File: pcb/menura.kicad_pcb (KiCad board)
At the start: 2 copper layers, 128.1 x 103.8 mm, 54 parts, among them SW1 SW_Push, SW10 SW_Push, SW11 SW_Push, SW12 SW_Push, SW13 SW_Push, SW14 SW_Push, SW15 SW_Push, SW16 SW_Push, SW17 SW_Push, SW18 SW_Push, SW19 SW_Push, SW2 SW_Push, SW20 SW_Push, SW21 SW_Push, SW22 SW_Push, SW3 SW_Push, SW4 SW_Push, SW5 SW_Push, SW6 SW_Push, SW7 SW_Push, SW8 SW_Push, SW9 SW_Push

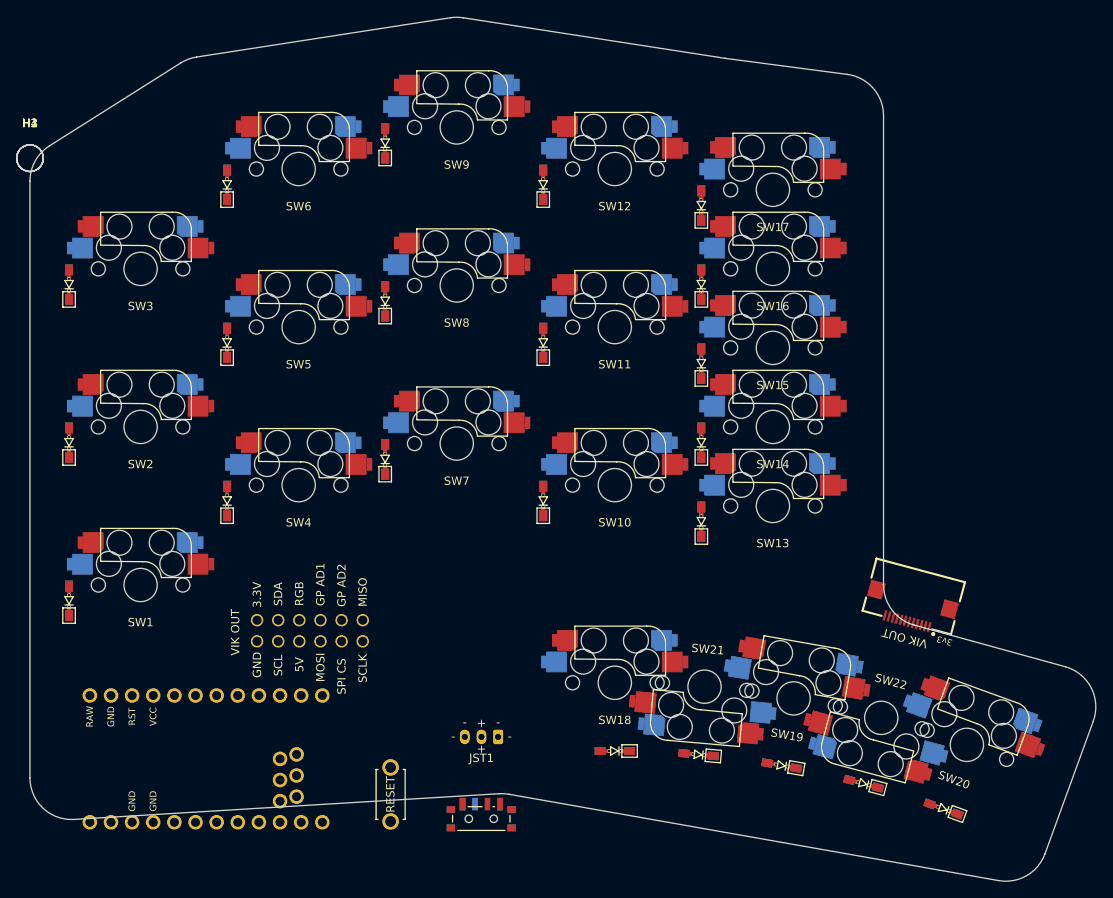
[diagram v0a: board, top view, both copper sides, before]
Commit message: edge cut wip
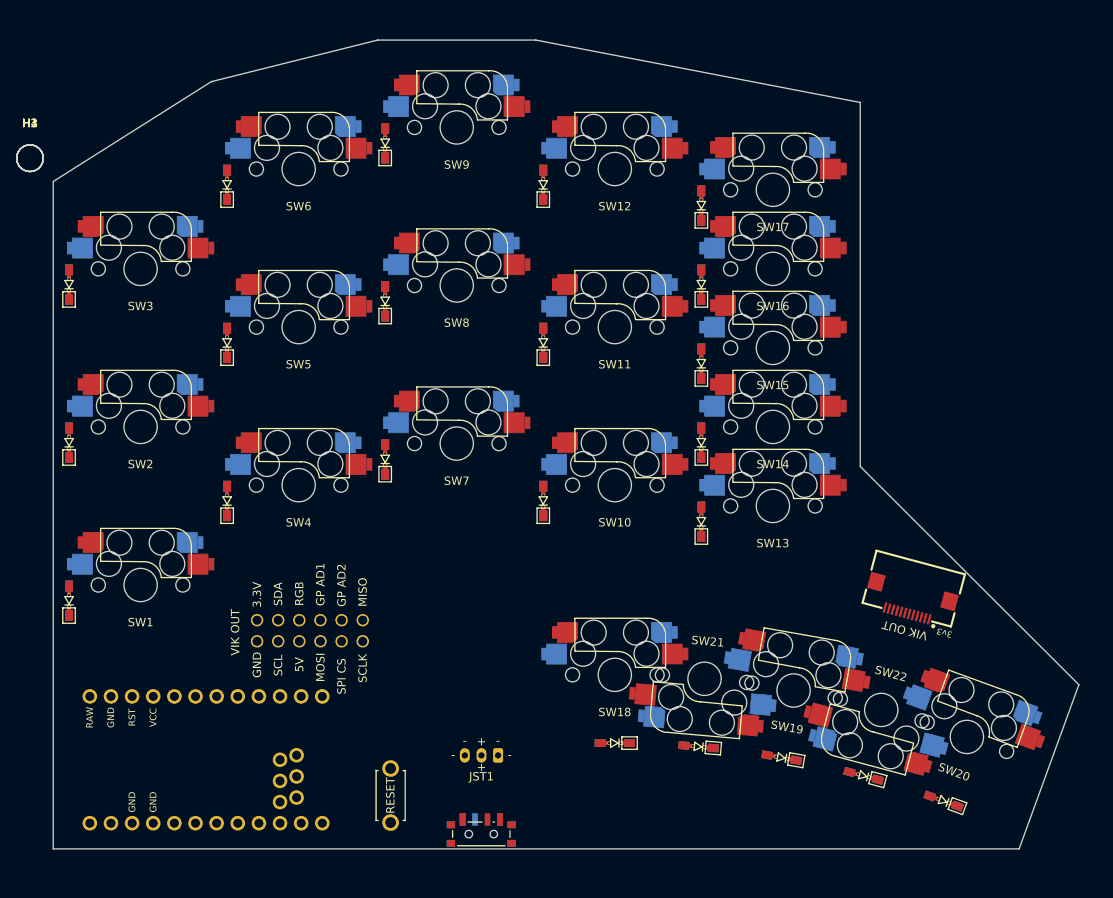
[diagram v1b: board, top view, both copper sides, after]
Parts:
- moved JST1 2.22 mm to (140.9, 118.0)
- moved PWR1 1.84 mm to (140.9, 129.9)
- moved D18 0.95 mm to (157.0, 119.0)
- moved D21 0.95 mm to (167.1, 119.4)
- moved D22 0.95 mm to (186.9, 122.9)
- moved SW18 0.95 mm to (157.0, 110.8)
- moved SW20 0.95 mm to (199.3, 118.3)
- moved D19 0.95 mm to (177.1, 120.8)
- moved D20 0.95 mm to (196.5, 126.0)
- moved SW19 0.95 mm to (178.5, 112.7)
- moved SW21 0.95 mm to (167.8, 111.3)
- moved SW22 0.95 mm to (189.0, 115.0)
- moved VIK1 0.95 mm to (192.7, 101.4)
- moved RSW1 0.13 mm to (130.1, 125.3)
- moved MCU1 0.11 mm to (107.0, 120.6)
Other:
- board size 128.1 x 103.8 mm -> 123.3 x 97.2 mm
